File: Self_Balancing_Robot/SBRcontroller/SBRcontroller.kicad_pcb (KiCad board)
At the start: 2 copper layers, 113.5 x 60.8 mm, 25 parts, among them J1 Screw_Terminal_01x02, J4 OLED SCREEN, U1 THB001P, U11 THB001P, U2 MX1A-11NN, U3 MX1A-11NN, U4 MX1A-11NN, U6 NRF24L01_Breakout

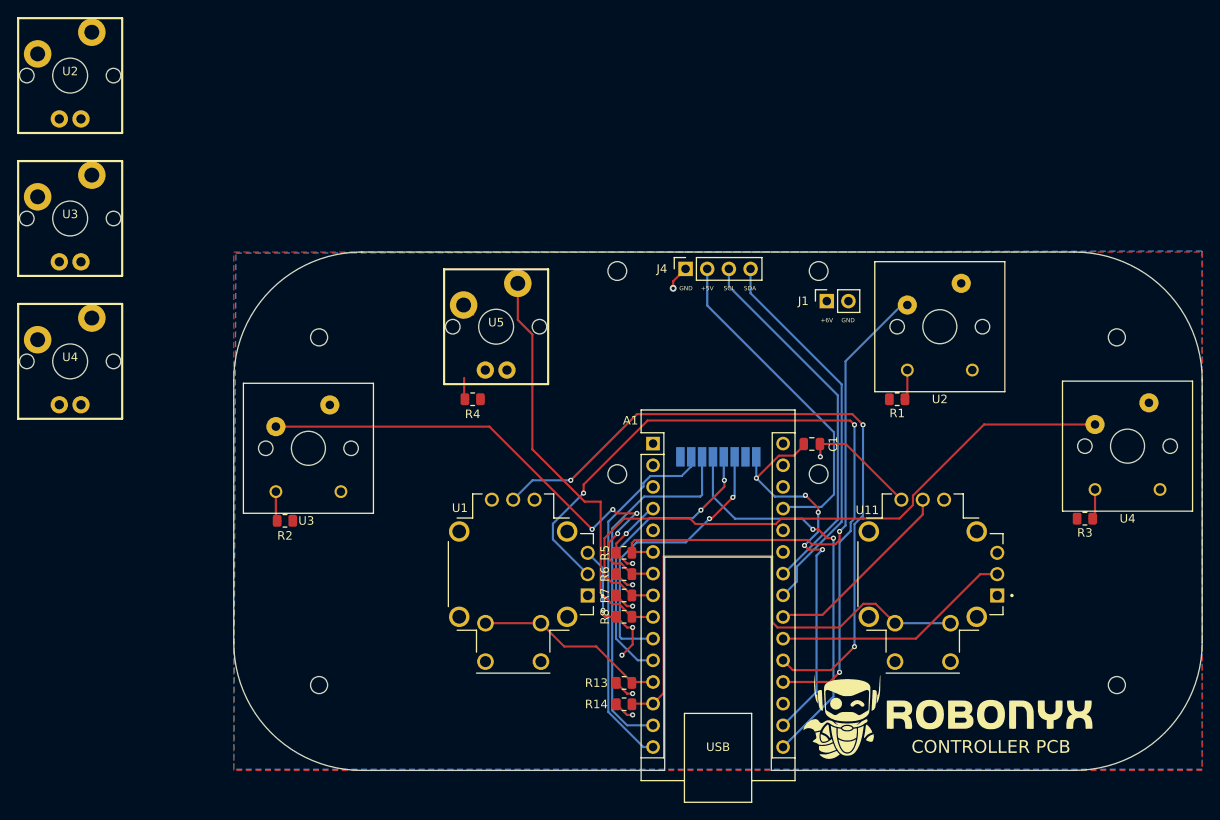
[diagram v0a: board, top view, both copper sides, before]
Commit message: sbrcotnrollerm update from windows laptop
dcefefefefe
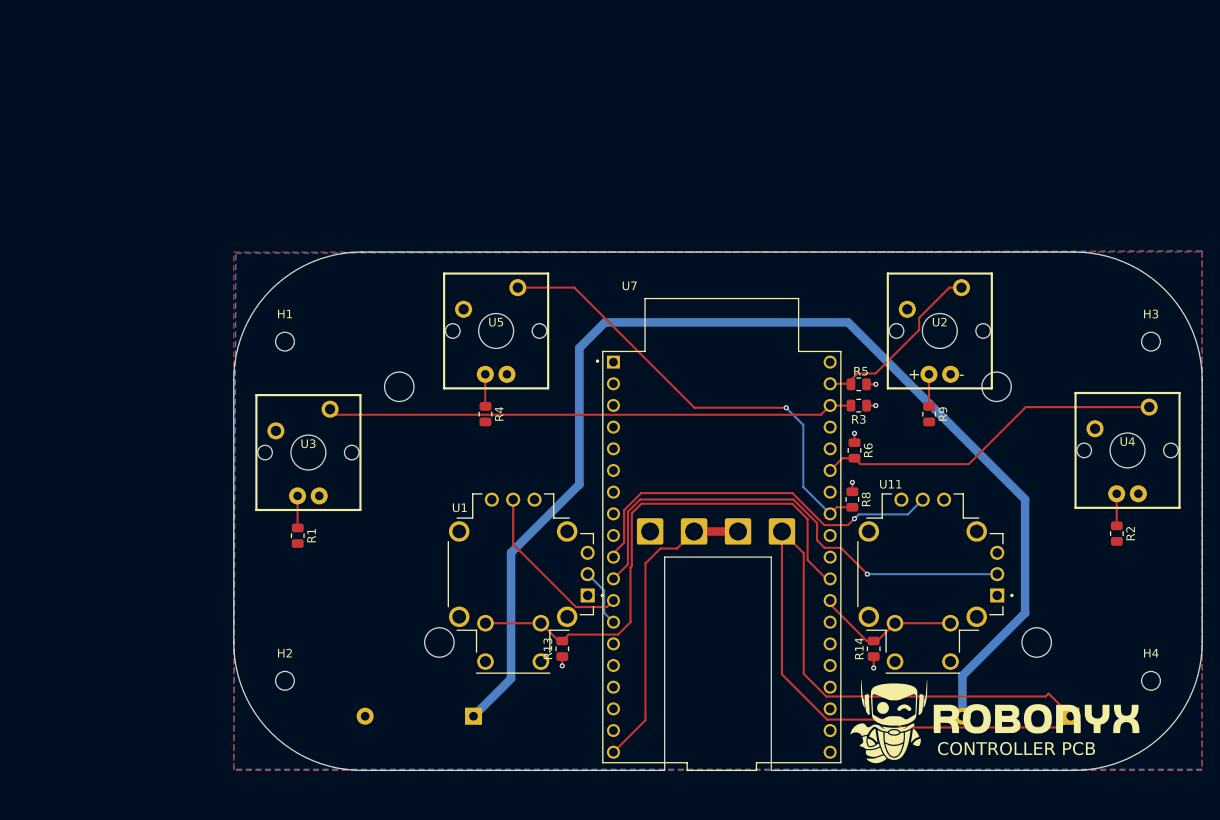
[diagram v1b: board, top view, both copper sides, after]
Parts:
- removed A1: Arduino_Nano_v3.x, Module:Arduino_Nano
- removed C1: 10UF, Capacitor_SMD:C_0805_2012Metric
- removed J1: Screw_Terminal_01x02, Connector_PinSocket_2.54mm:PinSocket_1x02_P2.54mm_Vertical
- removed R7: 10K, Resistor_SMD:R_0805_2012Metric
- removed the U2 at (126.0, 80.0)
- removed the U3 at (52.0, 94.2)
- removed the U4 at (148.0, 94.0)
- removed U6: NRF24L01_Breakout, nRF24L01BRKT_SMD:nRF24L01_Breakout_SMD
- added BT1: Battery_Cell, Battery:BatteryHolder_Keystone_2468_2xAAA, B.Cu at (141.3, 125.7)
- added BT2: Battery_Cell, Battery:BatteryHolder_Keystone_2468_2xAAA, B.Cu at (71.3, 125.7)
- added H1: MountingHole, MountingHole:MountingHole_2.2mm_M2, F.Cu at (49.2, 81.8)
- added H2: MountingHole, MountingHole:MountingHole_2.2mm_M2, F.Cu at (49.2, 121.5)
- added H3: MountingHole, MountingHole:MountingHole_2.2mm_M2, F.Cu at (150.8, 81.8)
- added H4: MountingHole, MountingHole:MountingHole_2.2mm_M2, F.Cu at (150.8, 121.5)
- added J2: -SW, Connector_Wire:SolderWire-1.5sqmm_1x01_D1.7mm_OD3mm, B.Cu at (107.5, 104.0)
- added J3: +SW, Connector_Wire:SolderWire-1.5sqmm_1x01_D1.7mm_OD3mm, B.Cu at (102.3, 104.0)
- added J5: -SWLED, Connector_Wire:SolderWire-1.5sqmm_1x01_D1.7mm_OD3mm, B.Cu at (92.0, 104.0)
- added R9: 330R, Resistor_SMD:R_0805_2012Metric, F.Cu at (124.8, 90.2)
- added U7: ESP32-DEVKITC, ESP32-DEVKITC:MODULE_ESP32-DEVKITC, F.Cu at (100.5, 107.0)
- J4: value OLED SCREEN -> +SWLED; footprint Connector_PinSocket_2.54mm:PinSocket_1x04_P2.54mm_Vertical -> Connector_Wire:SolderWire-1.5sqmm_1x01_D1.7mm_OD3mm; moved to B.Cu
- R1, R2, R4: value 68R -> 330R
- R3: value 68R -> 10K
- U2, U3, U4, U5: footprint Button_Switch_Keyboard:SW_Cherry_MX_3mmLED -> MX1A-11NN:Cherry_MX_3mmLED
- moved U4 124.3 mm to (148.0, 94.0)
- moved U2 106.1 mm to (126.0, 80.0)
- moved R2 97.5 mm to (146.8, 104.2), turned to -90 degrees
- moved R1 72.0 mm to (50.8, 104.5), turned to -90 degrees
- moved U3 38.8 mm to (52.0, 94.2)
- moved R5 33.9 mm to (116.5, 86.8), turned to 180 degrees
- moved J4 30.8 mm to (97.2, 104.0), turned to -90 degrees
- moved R6 30.6 mm to (116.0, 94.5), turned to -90 degrees
- moved R8 30.1 mm to (115.8, 100.2), turned to -90 degrees
- moved R14 30.0 mm to (118.2, 117.8), turned to 90 degrees
- moved R3 29.6 mm to (116.5, 89.2)
- moved R13 8.28 mm to (81.8, 117.8), turned to 90 degrees
- moved G*** 5.52 mm to (132.5, 126.0)
- moved R4 2.30 mm to (72.8, 90.2), turned to -90 degrees
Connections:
- net Net-(A1-D10) renamed /SW2
- net Net-(A1-D3) renamed /KB1
- net Net-(A1-D6) renamed /KB4
- net Net-(A1-D9) renamed /SW1
- J4 pad 1: GND -> +6V
- R1 pad 2: +6V -> +3V3
- R2 pad 1: Net-(U3-A) -> Net-(R2-Pad1)
- R2 pad 2: +6V -> +3V3
- R3 pad 1: Net-(U4-A) -> GND
- R3 pad 2: +6V -> /KB2
- R4 pad 1: Net-(U5-A) -> Net-(R4-Pad1)
- R4 pad 2: +6V -> +3V3
- R6 pad 2: Net-(A1-D4) -> /KB3
- U1 pad C: +6V -> +3V3
- U1 pad D: +6V -> +3V3
- U1 pad VR1_1: +6V -> +3V3
- U1 pad VR1_2: Net-(A1-A0) -> /P1V
- U1 pad VR2_1: +6V -> +3V3
- U1 pad VR2_2: Net-(A1-A1) -> /P1H
- U11 pad C: +6V -> +3V3
- U11 pad D: +6V -> +3V3
- U11 pad VR1_1: +6V -> +3V3
- U11 pad VR1_2: Net-(A1-A2) -> /P2V
- U11 pad VR2_1: +6V -> +3V3
- U11 pad VR2_2: Net-(A1-A3) -> /P2H
- U2 pad A: GND -> Net-(R9-Pad1)
- U2 pad K: Net-(R1-Pad1) -> GND
- U2 pad S1: +6V -> +3V3
- U3 pad A: GND -> Net-(R1-Pad1)
- U3 pad K: Net-(R2-Pad1) -> GND
- U3 pad S1: +6V -> +3V3
- U3 pad S2: Net-(A1-D4) -> /KB2
- U4 pad A: GND -> Net-(R2-Pad1)
- U4 pad K: Net-(R4-Pad1) -> GND
- U4 pad S1: +6V -> +3V3
- U4 pad S2: Net-(A1-D5) -> /KB3
- U5 pad A: GND -> Net-(R4-Pad1)
- U5 pad K: Net-(R7-Pad1) -> GND
- U5 pad S1: +6V -> +3V3
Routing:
- net Net-(BT1--): track 0.00 -> 138.8 mm
- net Net-(BT1-+): track 0.00 -> 105.1 mm
- net Net-(A1-A0): track 85.6 -> 0.00 mm, vias 3 -> 0
- net Net-(A1-A1): track 82.1 -> 0.00 mm, vias 3 -> 0
- net Net-(A1-D5): track 75.2 -> 0.00 mm
- net /KB2: track 0.00 -> 61.5 mm
- net Net-(A1-D4): track 61.0 -> 0.00 mm, vias 4 -> 0
- net Net-(A1-Pad6): track 59.8 -> 0.00 mm, vias 1 -> 0
- net /P2V: track 0.00 -> 57.2 mm, vias 0 -> 1
- net +3.3V: track 48.3 -> 0.00 mm, vias 5 -> 0
- net Net-(A1-D13): track 47.7 -> 0.00 mm, vias 2 -> 0
- net /SW2: track 64.0 -> 17.4 mm
- net /SDA: track 45.5 -> 0.00 mm
- net GND: track 51.8 -> 6.78 mm, vias 11 -> 6
- net /P2H: track 0.00 -> 44.8 mm, vias 0 -> 1
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- added copper zone on F.Cu, net +3V3
- removed copper zone on F.Cu, net +6V
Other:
- outline, holes or cut-outs redrawn
- board text added: "+SW"
- board text added: "+SWLED"
- board text added: "-SW"
- board text added: "-SWLED"
- board text removed: "+5V"
- board text removed: "+6V"
- board text removed: "GND"
- board text removed: "SCL"
- board text removed: "SDA"
